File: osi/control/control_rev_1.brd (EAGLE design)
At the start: 25.4 x 25.4 mm, 12 parts, among them J1 1X2-3.5MM, J2 1X2-3.5MM

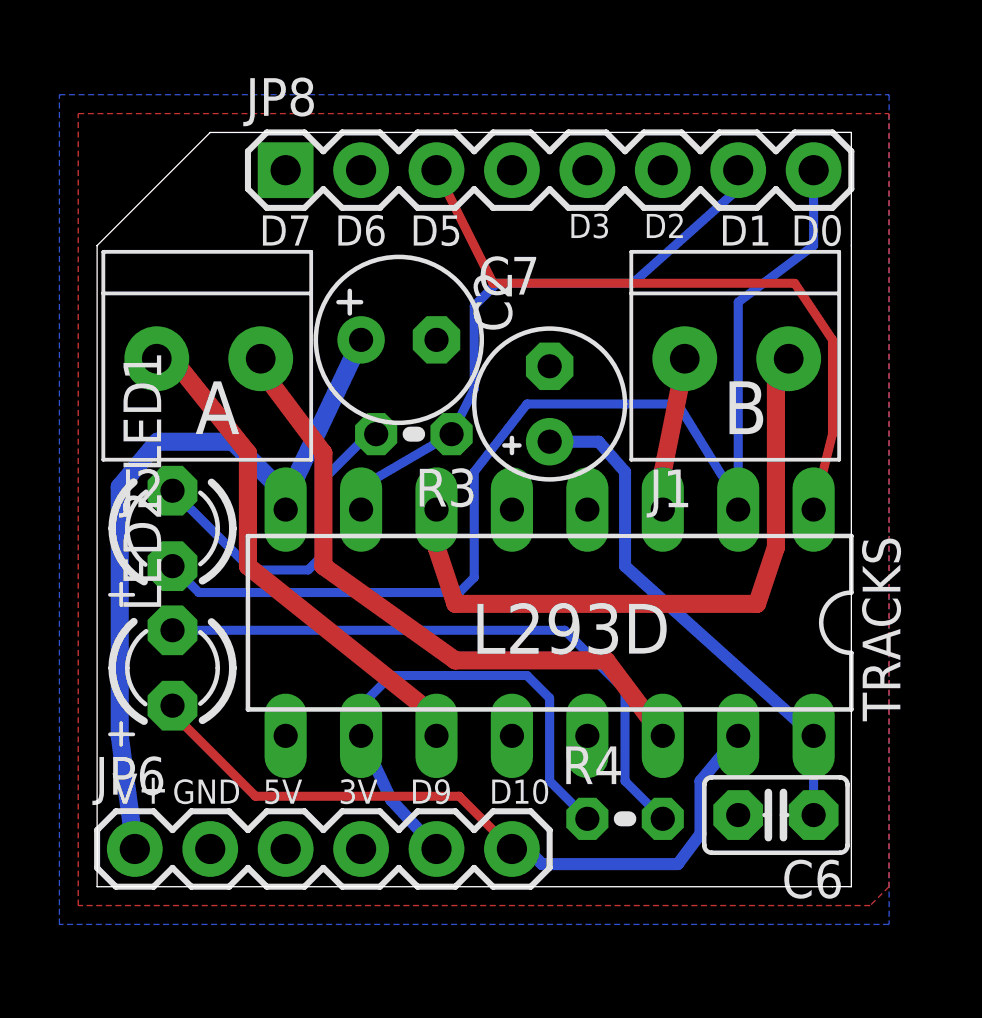
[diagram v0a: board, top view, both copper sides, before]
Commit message: control
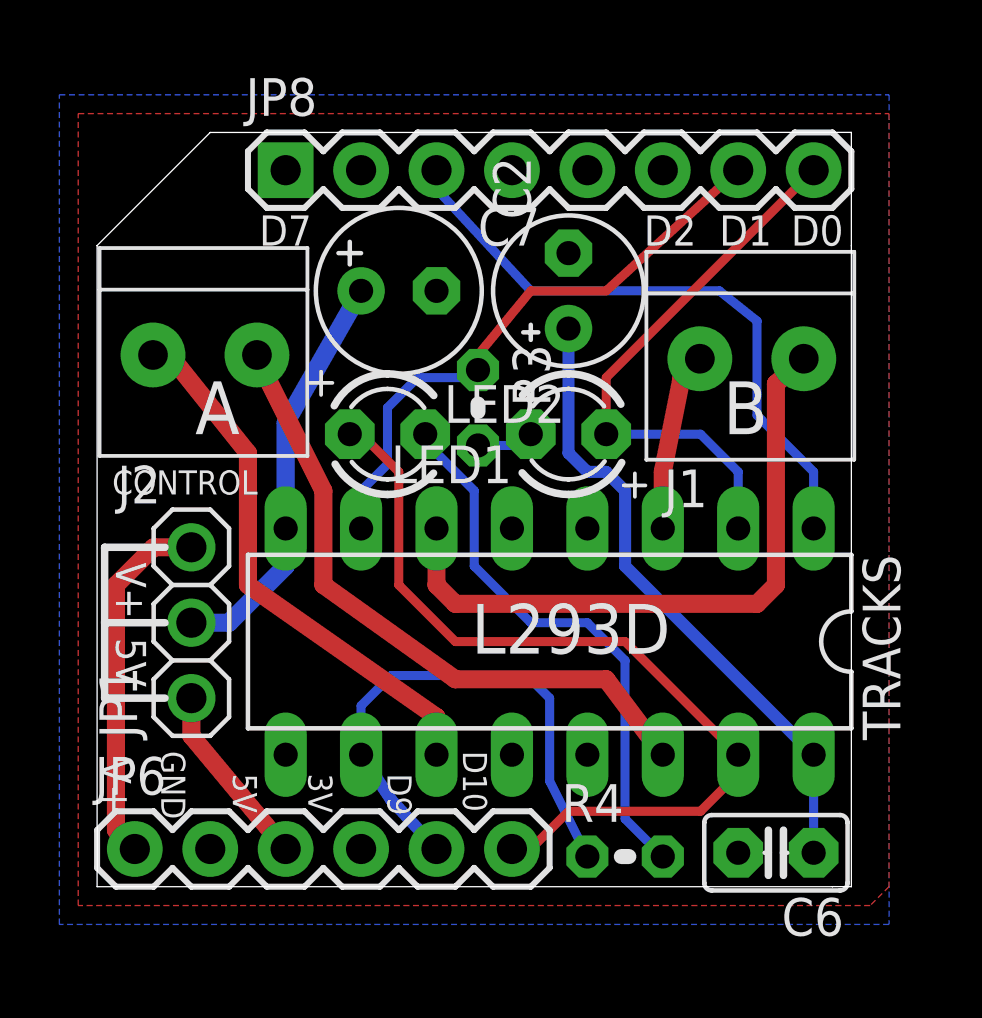
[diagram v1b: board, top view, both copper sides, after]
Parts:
- added JP1: (no value), adafruit_mod:1X03
- moved LED1 13.7 mm to (15.9, 15.2), turned to 180 degrees
- moved LED2 10.7 mm to (9.78, 15.2), turned to 0 degrees
- moved C2 3.86 mm to (15.9, 20.1)
- moved R3 2.33 mm to (12.8, 16.1), turned to 270 degrees
- moved C7 1.65 mm to (10.2, 20.1)
- moved R4 1.27 mm to (17.8, 1.02)
- moved C6 1.27 mm to (22.9, 1.14)
- moved TRACKS 0.63 mm to (15.2, 8.26)
- moved J1 0.51 mm to (22.1, 17.8)
- moved J2 0.18 mm to (3.68, 17.9)
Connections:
- new net N$8: C7.+, JP1.2, TRACKS.8
- net +5V: now also JP1.1
- net V+: now also JP1.3; no longer C7.+, TRACKS.8
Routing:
- net AREF_D0: track 38.8 -> 18.7 mm
- net V+: track 27.1 -> 12.2 mm
- net N$8: track 0.00 -> 13.9 mm
- net N$6: track 11.3 -> 1.94 mm
- net +5V: track 0.00 -> 6.23 mm
- net D10: track 24.4 -> 29.1 mm
- net VCC: track 17.4 -> 21.4 mm
- net N$7: track 20.9 -> 18.7 mm
- net D5: track 22.5 -> 21.1 mm
- net D9: track 17.3 -> 18.4 mm
- net N$1: track 5.19 -> 6.29 mm
- net N$4: track 17.2 -> 18.2 mm
- net N$2: track 21.4 -> 22.1 mm
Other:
- board text added: "D4"
- board text removed: "One Square Inch"
